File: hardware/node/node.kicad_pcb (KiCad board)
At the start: 2 copper layers, 27.1 x 45 mm, 56 parts, among them J1 USB_C_Receptacle_USB2.0_14P, J2 SWD, J3 Batt, J4 Solar, Q1 8205A_C2762931, U1 VGDD79S868N0S1, U2 MS88SF3-NRF52840, U3 SRV05-4, U4 TP4056-42-ESOP8, U5 DW01A, U6 ME6217C33M5G, U7 CN3163

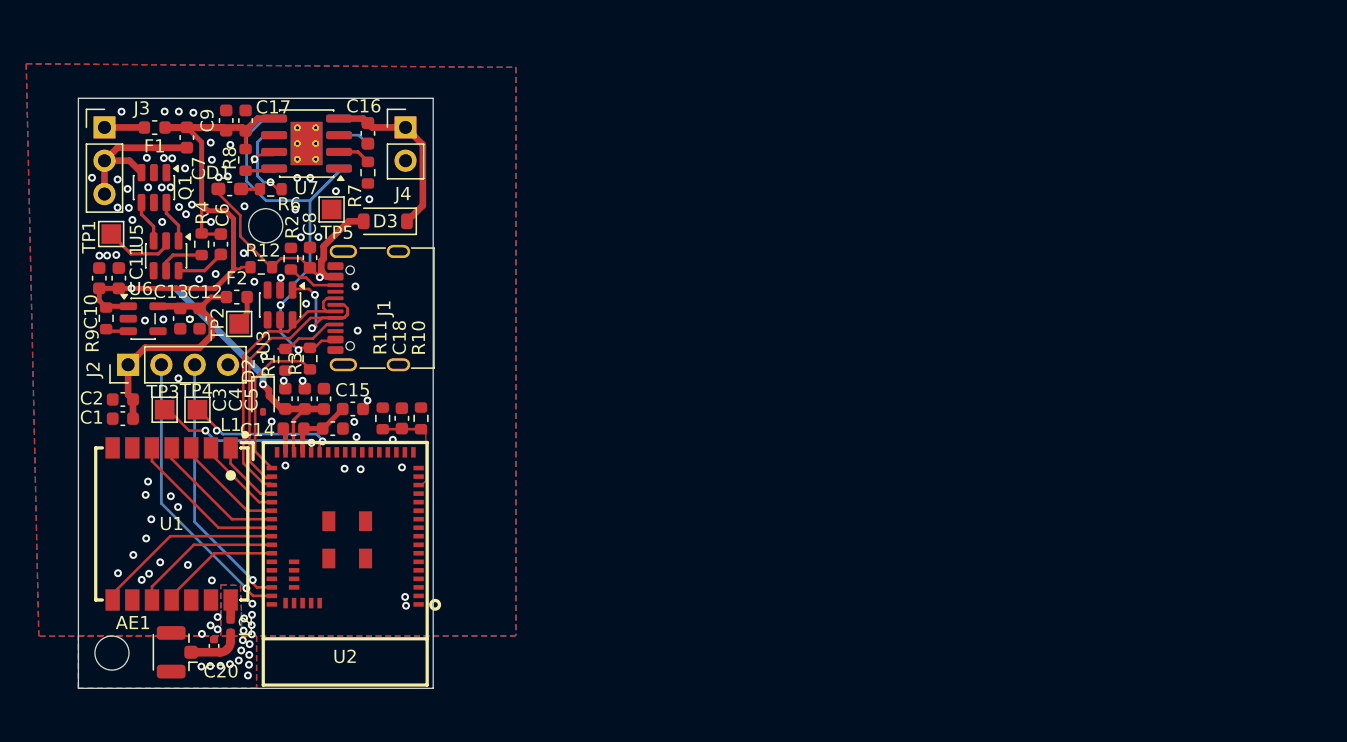
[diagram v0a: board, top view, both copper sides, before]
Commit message: a
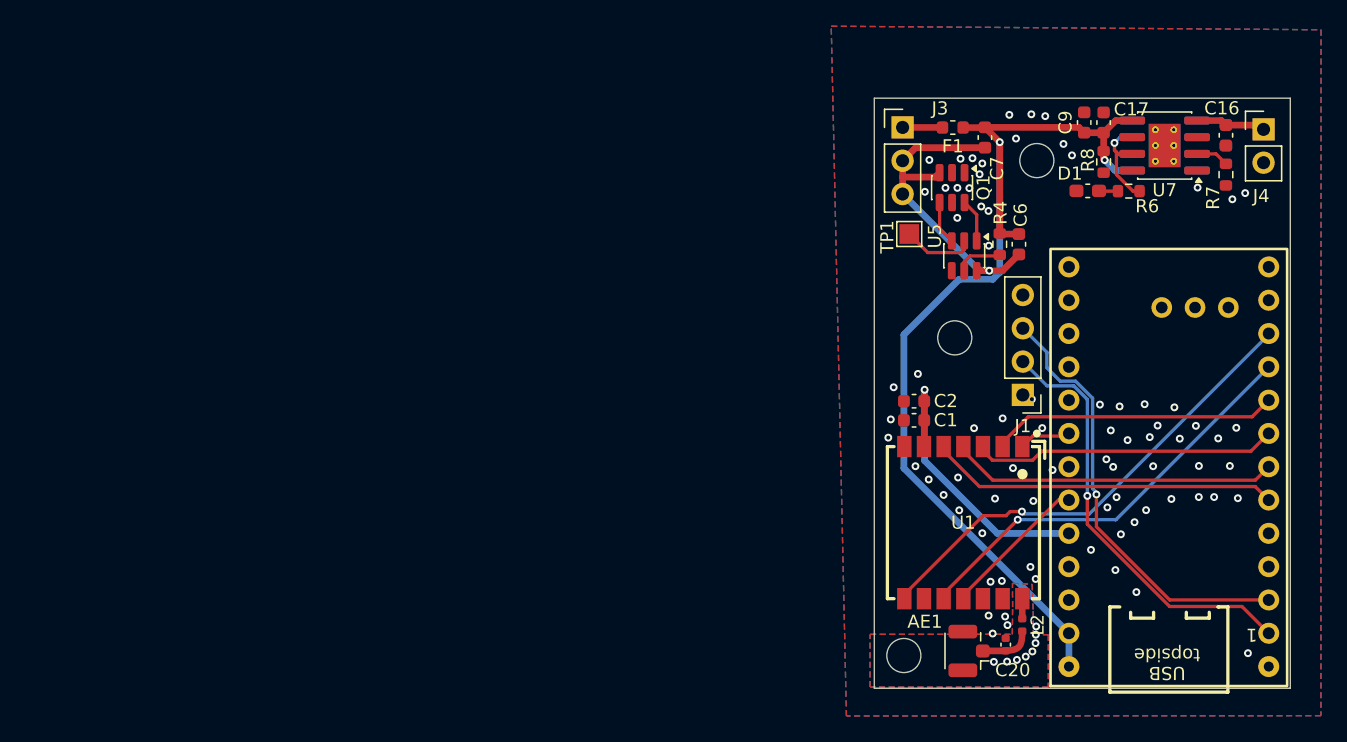
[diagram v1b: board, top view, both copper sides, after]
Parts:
- removed C10, C11, C12, C13, C15, C4, C5: 10u, Capacitor_SMD:C_0603_1608Metric
- removed C14, C18, C3, C8: 100n, Capacitor_SMD:C_0603_1608Metric
- removed D2: TPGC03C-A, Diode_SMD:D_SOD-323
- removed D3: 1N4148W, Diode_SMD:D_SOD-123
- removed F2: Polyfuse, Fuse:Fuse_0603_1608Metric
- removed J2: SWD, Connector_PinHeader_2.54mm:PinHeader_1x04_P2.54mm_Vertical
- removed L1: 10u 80ma+, Inductor_SMD:L_0603_1608Metric
- removed R1, R2: 5.1k, Resistor_SMD:R_0603_1608Metric
- removed R10, R11, R9: 1M, Resistor_SMD:R_0603_1608Metric
- removed R12, R3: 0r, Resistor_SMD:R_0603_1608Metric
- removed TP2, TP3, TP4, TP5: TestPoint, TestPoint:TestPoint_Pad_1.5x1.5mm
- removed U3: SRV05-4, Package_TO_SOT_SMD:SOT-23-6
- removed U6: ME6217C33M5G, Package_TO_SOT_SMD:SOT-23-5
- J1: value USB_C_Receptacle_USB2.0_14P -> Conn_01x04; footprint Connector_USB:USB_C_Receptacle_G-Switch_GT-USB-7010ASV -> Connector_PinHeader_2.54mm:PinHeader_1x04_P2.54mm_Vertical
- U2: value MS88SF3-NRF52840 -> nice_nano; footprint easyeda2kicad:BULETM-SMD_MS88SF3_V1.0 -> library:SuperMini NRF52840
- moved U2 71.2 mm to (213.6, 138.3)
- moved C16 65.4 mm to (210.3, 97.8)
- moved R5 65.4 mm to (210.3, 97.8)
- moved R7 65.4 mm to (210.3, 100.8)
- moved C17 65.4 mm to (201.0, 96.8)
- moved C9 65.4 mm to (199.5, 96.8)
- moved D1 65.4 mm to (199.8, 102.0)
- moved J4 65.4 mm to (213.2, 97.3)
- moved R6 65.4 mm to (202.9, 102.1)
- moved R8 65.4 mm to (201.0, 99.8)
- moved U4 65.4 mm to (205.7, 98.6)
- moved U7 65.4 mm to (205.7, 98.6)
- moved C6 60.9 mm to (194.5, 106.1)
- moved F1 60.9 mm to (189.5, 97.2)
- moved Q1 60.9 mm to (189.4, 101.8)
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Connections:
- U2 pad 1: GND -> /sdl
- U2 pad 10: unconnected-(U2-P0.29-Pad10) -> /dio3
- U2 pad 13: unconnected-(U2-P0.31-Pad13) -> +BATT
- U2 pad 14: unconnected-(U2-P0.27-Pad14) -> GND
- U2 pad 15: /batt_sens -> unconnected-(U2-RST-Pad15)
- U2 pad 16: unconnected-(U2-P0.04-Pad16) -> +3V3
- U2 pad 17: unconnected-(U2-P0.26-Pad17) -> /busy
- U2 pad 18: GND -> unconnected-(U2-P0.29-Pad18)
- U2 pad 19: unconnected-(U2-P0.07-Pad19) -> /rst
- U2 pad 2: unconnected-(U2-P1.11-Pad2) -> /scl
- U2 pad 28: unconnected-(U2-P0.18-Pad28) -> GND
- U2 pad 29: /scl -> +BATT
- U2 pad 3: unconnected-(U2-P1.12-Pad3) -> GND
- U2 pad 4: unconnected-(U2-P1.10-Pad4) -> GND
- U2 pad 5: unconnected-(U2-P1.14-Pad5) -> /cs
- U2 pad 6: unconnected-(U2-P0.03-Pad6) -> /clk
- U2 pad 7: unconnected-(U2-P1.13-Pad7) -> /mosi
- U2 pad 8: unconnected-(U2-P1.15-Pad8) -> /miso
- U2 pad 9: unconnected-(U2-P0.02-Pad9) -> /dio1
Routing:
- net VBUS: track 58.5 -> 0.00 mm, vias 3 -> 0
- net /d-: track 28.3 -> 0.00 mm, vias 2 -> 0
- net /dio3: track 14.4 -> 36.6 mm, vias 0 -> 1
- net /d+: track 22.0 -> 0.00 mm
- net Net-(J2-Pin_2): track 22.0 -> 0.00 mm, vias 1 -> 0
- net /scl: track 11.6 -> 33.6 mm, vias 2 -> 1
- net /dio1: track 11.5 -> 32.3 mm, vias 0 -> 1
- net Net-(J2-Pin_3): track 20.1 -> 0.00 mm, vias 1 -> 0
- net /sdl: track 13.0 -> 32.9 mm, vias 2 -> 1
- net /miso: track 6.63 -> 21.9 mm
- net /mosi: track 8.43 -> 23.3 mm
- net /clk: track 10.4 -> 25.0 mm
- net /cs: track 12.3 -> 26.7 mm
- net Net-(U2-VBUS): track 12.4 -> 0.00 mm
- net -BATT: track 16.2 -> 24.9 mm, vias 0 -> 1
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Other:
- board size 27.1 x 45 mm -> 31.7 x 45 mm
- board text removed: "swclk"
- board text removed: "swdio"

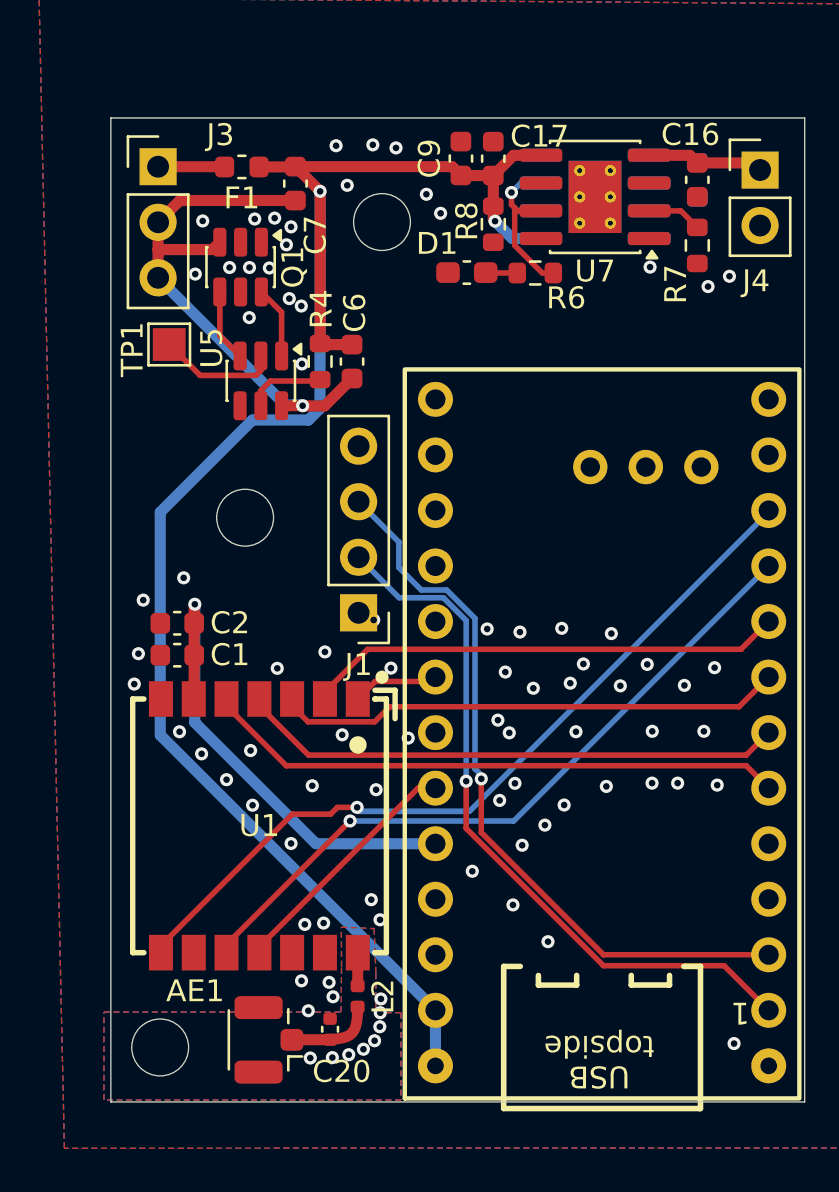
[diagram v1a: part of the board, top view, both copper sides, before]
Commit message: a
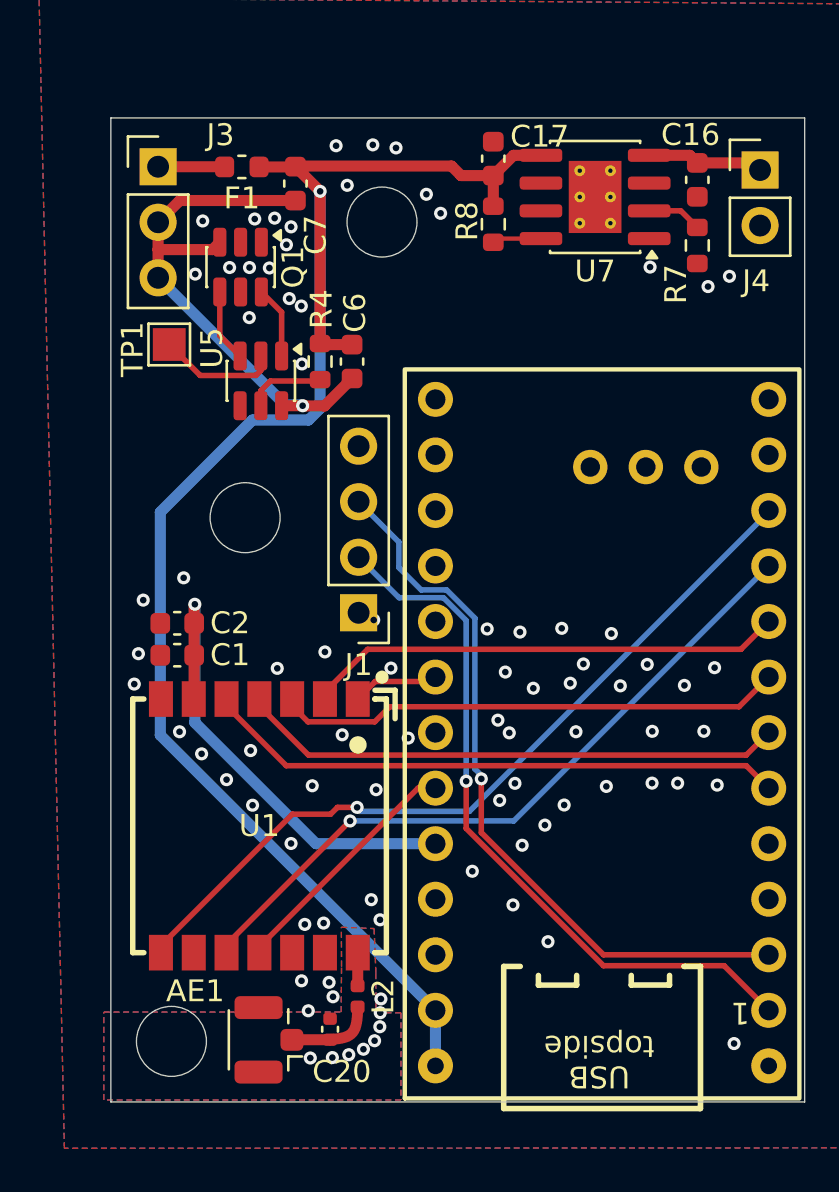
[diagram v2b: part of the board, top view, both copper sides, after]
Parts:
- removed C9: 10u, Capacitor_SMD:C_0603_1608Metric
- removed D1: LED, Capacitor_SMD:C_0603_1608Metric_Pad1.08x0.95mm_HandSolder
- removed R5: 10r, Resistor_SMD:R_0603_1608Metric
- removed R6: 1k, Resistor_SMD:R_0603_1608Metric
- removed U4: TP4056-42-ESOP8, Package_SO:SOIC-8-1EP_3.9x4.9mm_P1.27mm_EP2.41x3.3mm_ThermalVias
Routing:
- net /chrg: track 7.55 -> 0.00 mm, vias 1 -> 0
- net +BATT: track 77.8 -> 74.7 mm, vias 2 -> 1
- net Net-(U7-FB): track 0.00 -> 2.25 mm
- net Net-(D1-K): track 1.45 -> 0.00 mm
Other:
- outline, holes or cut-outs redrawn
